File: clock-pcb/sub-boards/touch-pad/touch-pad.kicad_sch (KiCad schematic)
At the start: 11 parts, among them J1 Conn_01x01_Pin, J2 Conn_01x01_Pin, J3 Conn_01x01_Pin, J4 Conn_01x01_Pin, J5 Conn_01x01_Pin, J6 Conn_01x01_Pin

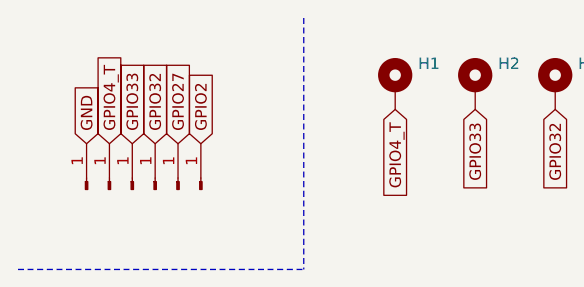
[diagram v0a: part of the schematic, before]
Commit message: touch slider pcb
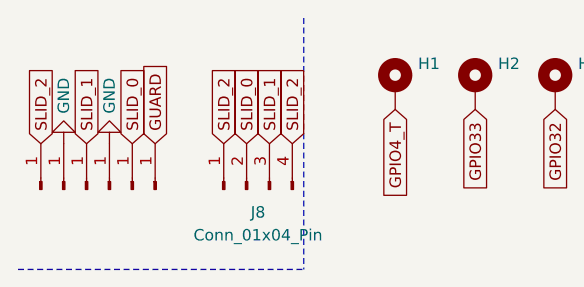
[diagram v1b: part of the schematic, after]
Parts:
- added J8: Conn_01x04_Pin, clock:TouchSlider-4_90x55mm, symbol Connector:Conn_01x04_Pin
- J6: footprint Connector_PinHeader_2.54mm:PinHeader_1x02_P2.54mm_Vertical_SMD_Pin1Left -> Connector_PinHeader_2.54mm:PinHeader_1x01_P2.54mm_Vertical
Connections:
- net GND: now also J1.1 (Pin_1), J3.1 (Pin_1); no longer J6.1 (Pin_1)
- net GPIO2: no longer J5.1 (Pin_1)
- net GPIO27: no longer J4.1 (Pin_1)
- net GPIO32: no longer J3.1 (Pin_1)
- net GPIO33: no longer J2.1 (Pin_1)
- net GPIO4_T: no longer J1.1 (Pin_1)
- new net GUARD: J5.1 (Pin_1)
- new net SLID_0: J4.1 (Pin_1), J8.2 (Pin_2)
- new net SLID_1: J2.1 (Pin_1), J8.3 (Pin_3)
- new net SLID_2: J6.1 (Pin_1), J8.1 (Pin_1), J8.4 (Pin_4)

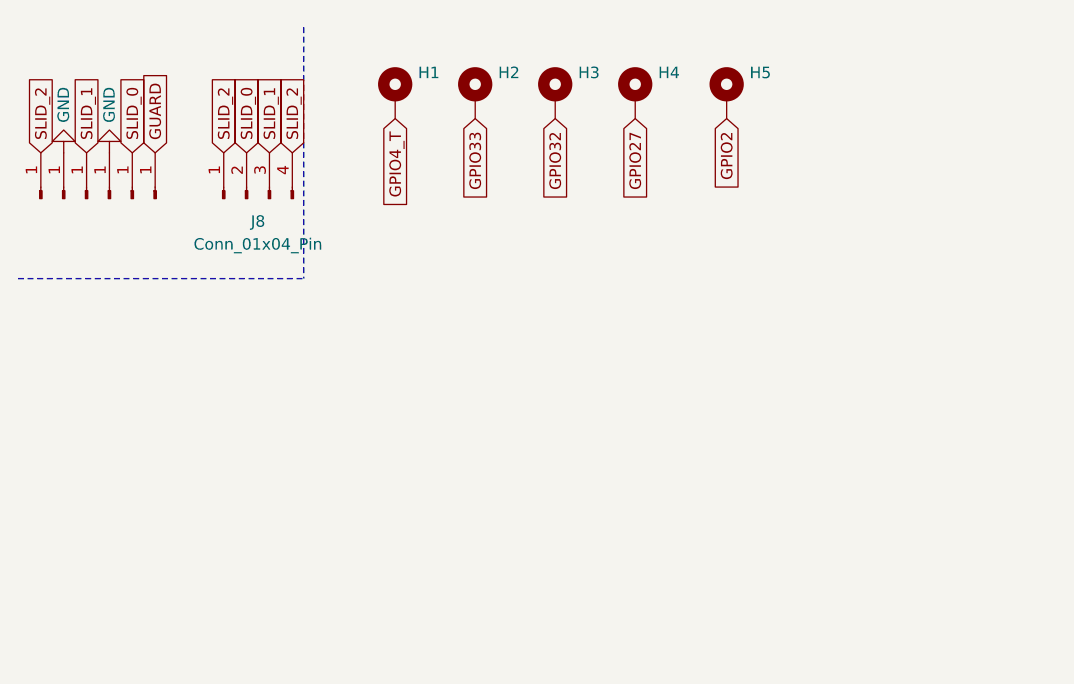
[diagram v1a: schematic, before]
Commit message: new pcb drafts
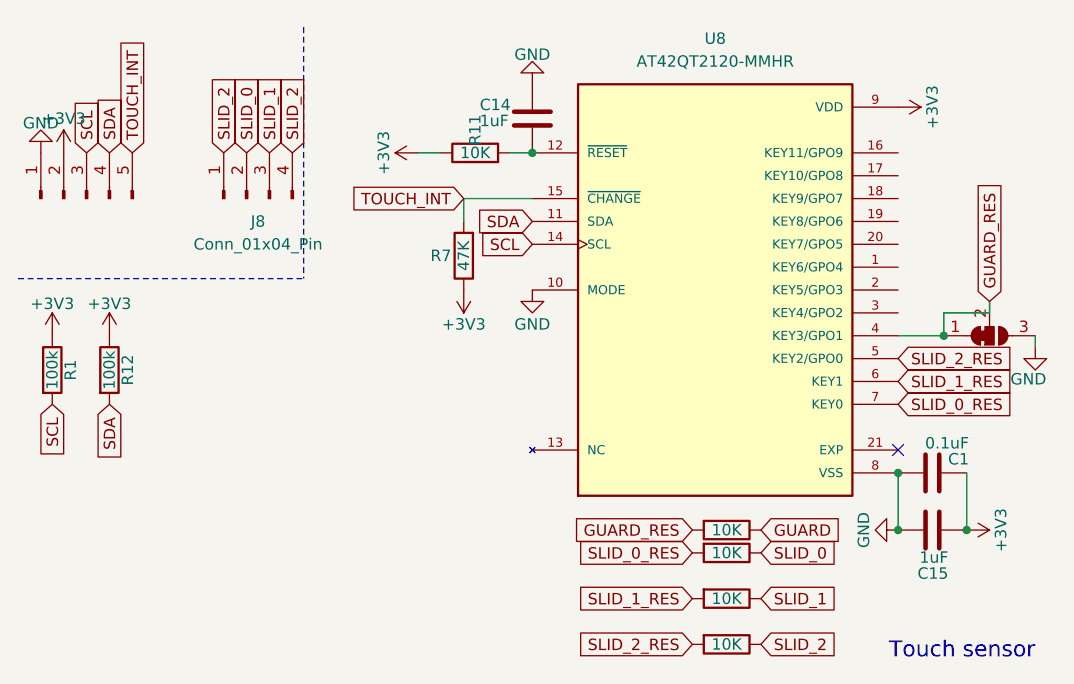
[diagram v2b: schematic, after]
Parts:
- removed H1, H2, H3, H4, H5: MountingHole_Pad_MP, symbol Mechanical:MountingHole_Pad_MP
- removed J1, J2, J3, J4, J5, J6: Conn_01x01_Pin, Connector_PinHeader_2.54mm:PinHeader_1x01_P2.54mm_Vertical, symbol Connector:Conn_01x01_Pin
- added C1: 0.1uF, Capacitor_SMD:C_0603_1608Metric, symbol Watchy:C
- added C14, C15: 1uF, Capacitor_SMD:C_0603_1608Metric, symbol Watchy:C
- added J7: Conn_01x05_Pin, Connector_PinHeader_2.54mm:PinHeader_1x05_P2.54mm_Vertical, symbol Connector:Conn_01x05_Pin
- added JP2: SolderJumper_3_Bridged12, clock:jumper_solder_small_3_bridged, symbol Jumper:SolderJumper_3_Bridged12
- added R1, R12: 100k, Resistor_SMD:R_0402_1005Metric, symbol Watchy:R
- added R10, R11, R16, R8, R9: 10K, Resistor_SMD:R_0402_1005Metric, symbol Watchy:R
- added R7: 47K, Resistor_SMD:R_0402_1005Metric, symbol Watchy:R
- added U8: AT42QT2120-MMHR, clock:QFN45P300X300X85-21N, symbol AT42QT2120-MMHR:AT42QT2120-MMHR
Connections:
- net GND: now also C1.1, C14.1, C15.1, J7.1 (Pin_1), JP2.3 (B), U8.10 (MODE), U8.8 (VSS)
- net GUARD: now also R9.1
- net SLID_0: now also R16.1
- net SLID_1: now also R10.1
- net SLID_2: now also R8.1
- new net: C14.2, R11.2, U8.12 (~{RESET})
- new net +3V3: C1.2, C15.2, J7.2 (Pin_2), R1.1, R11.1, R12.1, R7.1, U8.9 (VDD)
- new net GUARD_RES: JP2.1 (A), JP2.2 (C), R9.2, U8.4 (KEY3/GPO1)
- new net SCL: J7.3 (Pin_3), R1.2, U8.14 (SCL)
- new net SDA: J7.4 (Pin_4), R12.2, U8.11 (SDA)
- new net SLID_0_RES: R16.2, U8.7 (KEY0)
- new net SLID_1_RES: R10.2, U8.6 (KEY1)
- new net SLID_2_RES: R8.2, U8.5 (KEY2/GPO0)
- new net TOUCH_INT: J7.5 (Pin_5), R7.2, U8.15 (~{CHANGE})
- no-connect marks 0 -> 1
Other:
- note added: "Touch sensor"
